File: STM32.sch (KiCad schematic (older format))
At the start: 35 parts, among them U1 STM32H753IIKx, U4 FM25V02A-GTR, U9 USB3300-EZK-TR, Y1 16MHz, Y2 32.768, Y3 24MHz

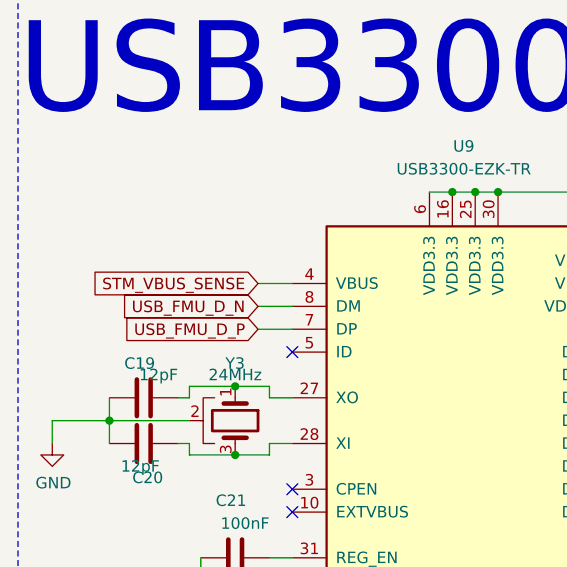
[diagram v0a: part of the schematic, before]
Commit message: working
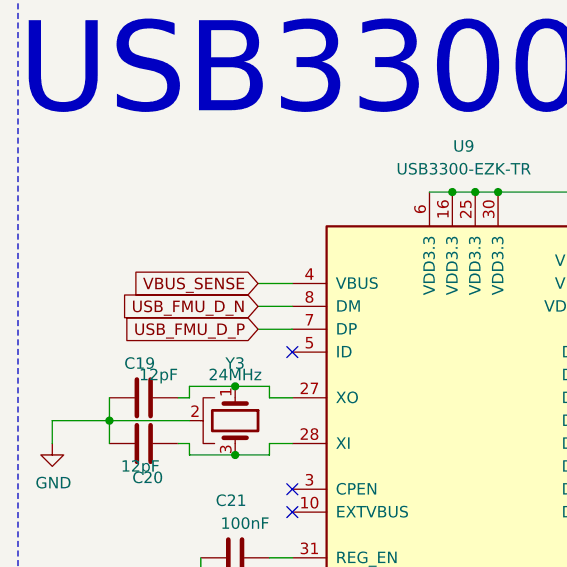
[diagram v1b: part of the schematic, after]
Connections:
- net STM_VBUS_SENSE is gone; now on net VBUS_SENSE: U9.4 (VBUS)
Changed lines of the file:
@@
 Wire Wire Line
 	2650 9000 2650 8850
-Text GLabel 2950 8850 2    50   Input ~ 0
-SENSORS_3V3
 Wire Wire Line
 	2950 8850 2650 8850
@@
 Wire Wire Line
 	3400 5650 3400 5750
-Text GLabel 1550 4150 0    50   Input ~ 0
-STM_VBUS_SENSE
 Text GLabel 1550 4250 0    50   Input ~ 0
 USB_FMU_D_N
@@
 Wire Wire Line
 	900  4750 900  4650
+Text GLabel 1550 4150 0    50   Input ~ 0
+VBUS_SENSE
+Text GLabel 2950 8850 2    50   Input ~ 0
+SENSORS_3V3
 $EndSCHEMATC
